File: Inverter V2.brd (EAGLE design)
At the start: 194.6 x 115.3 mm, 30 parts, among them Q1 ROHM_SCT3022ALGC11ROHM_SCT302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, Q2 ROHM_SCT3022ALGC11ROHM_SCT302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, Q3 ROHM_SCT3022ALGC11ROHM_SCT302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, Q4 ROHM_SCT3022ALGC11ROHM_SCT302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, Q5 ROHM_SCT3022ALGC11ROHM_SCT302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, Q6 ROHM_SCT3022ALGC11ROHM_SCT302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, U1 RASPBERRY_PICOTH

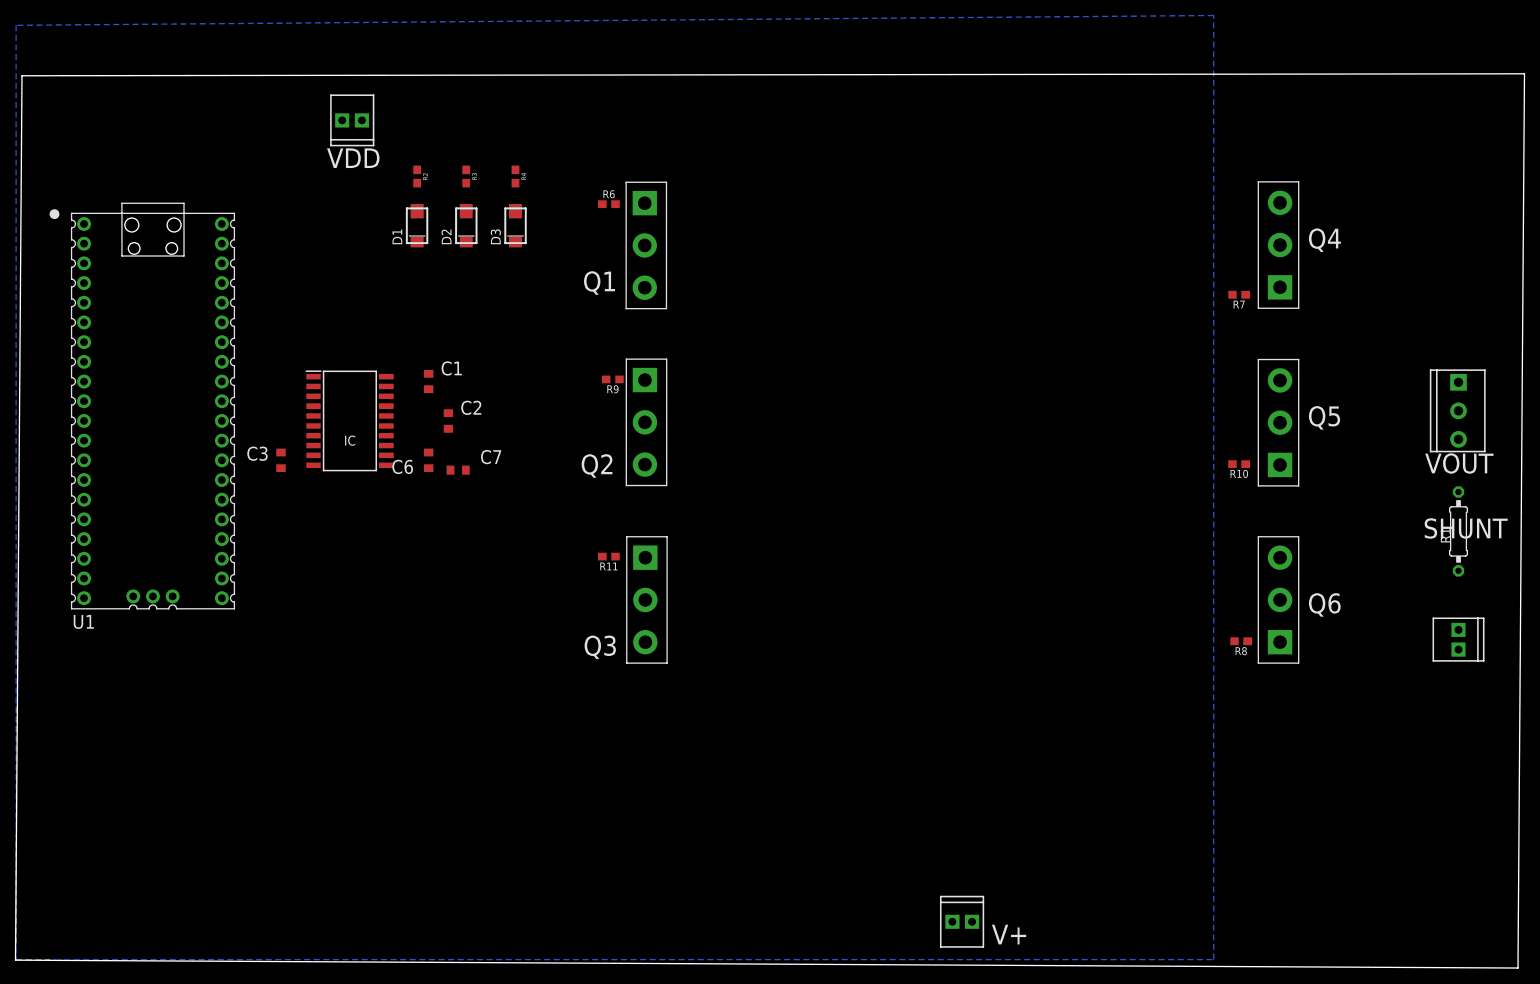
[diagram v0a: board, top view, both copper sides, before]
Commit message: Routing Inverter V2
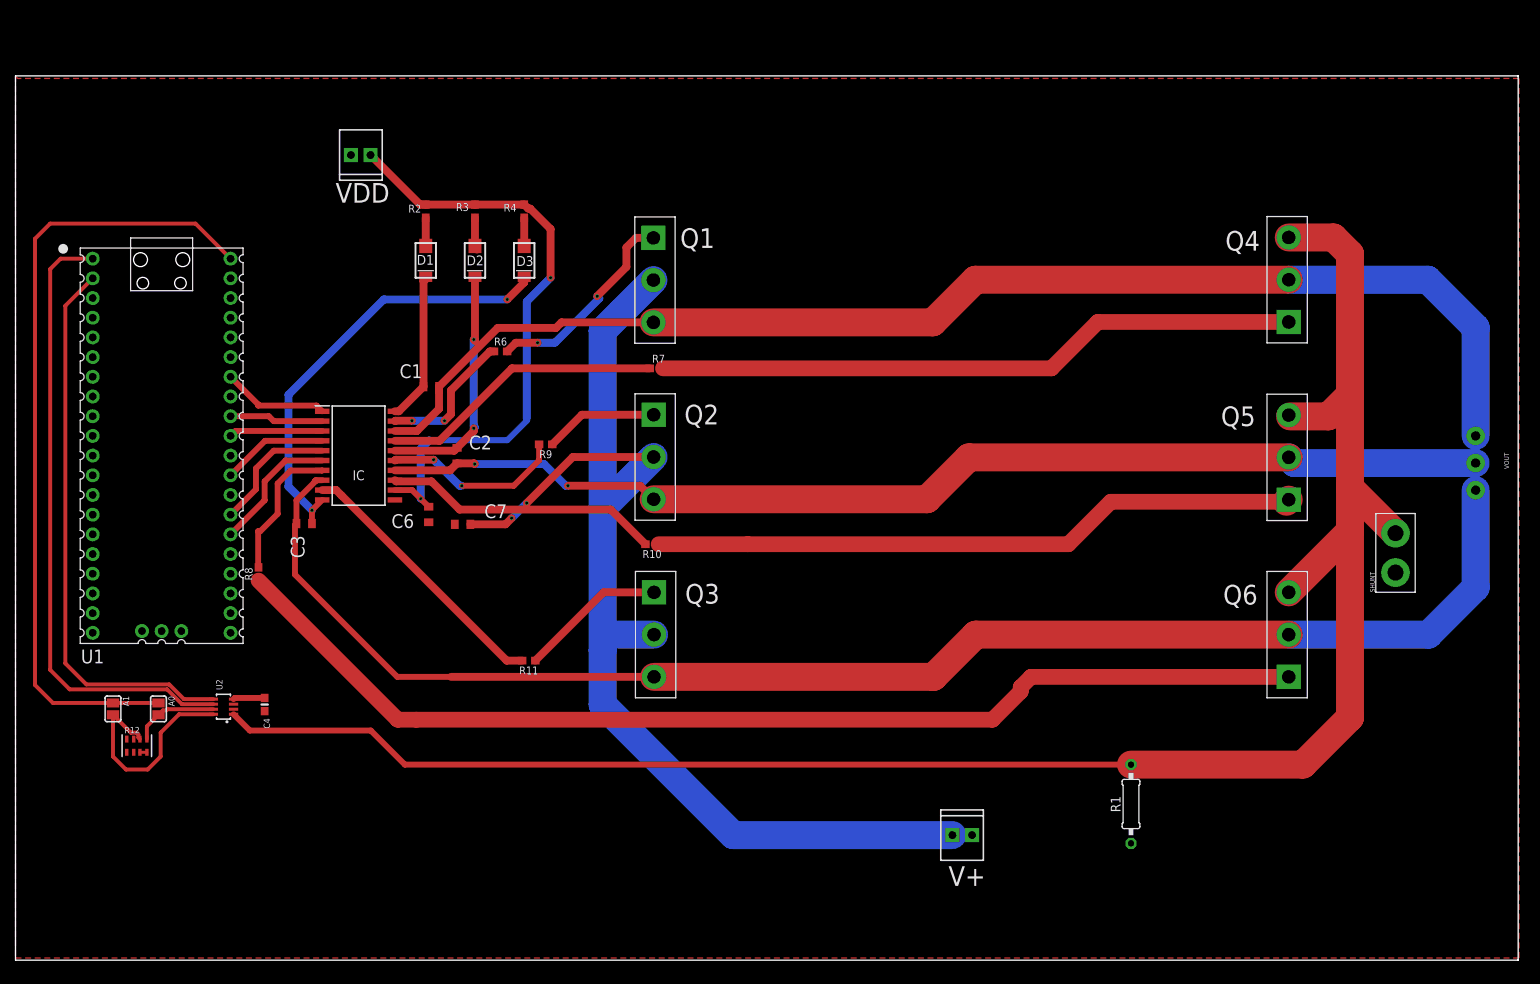
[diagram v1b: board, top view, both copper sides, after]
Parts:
- added A0, A1: (no value), microbuilder:SOLDERJUMPER_REFLOW_NOPASTE
- added C4: 0.1µF, microbuilder:0603-NO
- added R12: 10K, microbuilder:RESPACK_4X0603
- added U2: INA219BIDCNT, microbuilder:SOT23-8
- SHUNT: device SparkFun-Connectors:1X02_2.54_SCREWTERM -> SparkFun-Connectors:1X02_XTRA_BIG
- VOUT: device SparkFun-Connectors:SCREWTERMINAL-3.5MM-3_LOCK.007S -> SparkFun-Connectors:SCREWTERMINAL-3.5MM-3-NS
- moved R8 127.0 mm to (31.3, 49.8), turned to 270 degrees
- moved R10 76.4 mm to (82.1, 53.6)
- moved R7 75.8 mm to (82.7, 76.3)
- moved R1 55.0 mm to (143.9, 20.1), turned to 90 degrees
- moved R6 23.6 mm to (62.6, 78.5)
- moved R11 16.9 mm to (66.2, 38.6)
- moved SHUNT 12.8 mm to (178.0, 52.5), turned to 90 degrees
- moved R9 12.1 mm to (68.4, 66.5)
- moved V+ 11.2 mm to (120.8, 16.1)
- moved C3 8.69 mm to (37.2, 56.3), turned to 180 degrees
- moved VOUT 7.08 mm to (188.3, 67.6)
- moved C7 7.01 mm to (57.7, 56.2)
- moved C6 6.98 mm to (53.3, 57.5)
- moved Q2 4.61 mm to (82.5, 64.9)
- moved Q6 4.61 mm to (164.0, 42.0)
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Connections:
- net N$1 renamed HIN1
- net N$10 renamed VGIN3
- net N$11 renamed VGIN2
- net N$12 renamed HO3
- net N$14 renamed VGIN6
- net N$16 renamed VGIN4
- net N$2 renamed LO1
- net N$3 renamed LIN1
- net N$5 renamed LIN2
- net N$6 renamed VGIN1
- net N$7 renamed HIN3
- net N$8 renamed VGIN5
- net N$9 renamed LIN3
- removed net VBUS: U1.40
- new net ADDR0: A0.2, R12.5, U2.7
- new net ADDR1: A1.2, R12.6, U2.8
- new net SCL: U1.2, U2.5
- new net SDA: U1.1, U2.6
- new net VCC: A0.1, A1.1, C4.1, U1.40, U2.4
- net GND1: now also C4.2, R12.3, R12.4, SHUNT.1, U2.2, U2.3; no longer SHUNT.P1
- net SHUNT: now also SHUNT.2, U2.1; no longer SHUNT.P2
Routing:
- net SHUNT: track 0.00 -> 246.4 mm
- net VOUT3/VS3: track 0.00 -> 189.3 mm
- net VS1/VOUT1: track 0.00 -> 166.3 mm
- net V+: track 0.00 -> 153.6 mm, vias 0 -> 2
- net VS2/VOUT2: track 0.00 -> 144.2 mm, vias 0 -> 2
- net VGIN6: track 0.00 -> 142.9 mm
- net VCC: track 0.00 -> 106.4 mm
- net VGIN5: track 0.00 -> 83.6 mm
- net VGIN4: track 0.00 -> 83.2 mm
- net SDA: track 0.00 -> 80.6 mm
- net VDD: track 0.00 -> 80.0 mm, vias 0 -> 2
- net SCL: track 0.00 -> 72.1 mm
- net VB3: track 0.00 -> 56.9 mm, vias 0 -> 2
- net LO1: track 0.00 -> 36.7 mm
- net LO2: track 0.00 -> 35.7 mm
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- added copper zone on layer 1, net GND1
- removed copper zone on layer 16, net GND1
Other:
- board size 194.6 x 115.3 mm -> 193.8 x 114 mm
